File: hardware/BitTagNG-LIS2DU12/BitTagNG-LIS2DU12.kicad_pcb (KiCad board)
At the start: 2 copper layers, 17 x 9 mm, 22 parts, among them J201 CONN_02X04, J301 Conn_01x01, J302 Conn_01x01, J303 Conn_01x01, J304 Conn_01x01, J401 CONN_01X02, Q501 Q_NPN_BEC, U1 at25ex321D-UUN, U3 LIS2DW12TR, U302 stm32l431kc, U501 RV-3028-C7

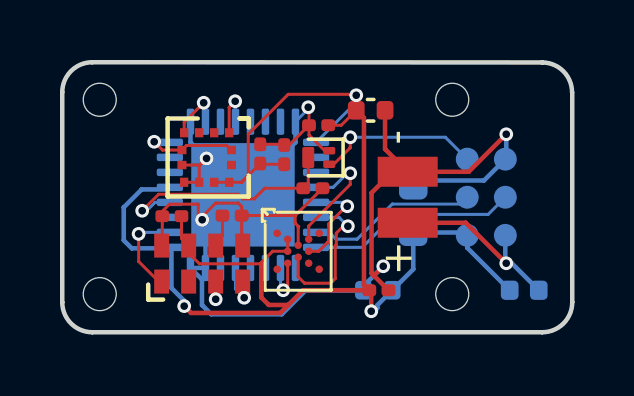
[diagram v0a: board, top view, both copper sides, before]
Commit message: update design
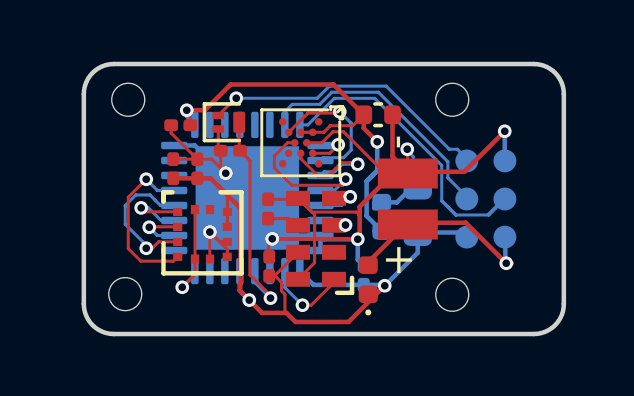
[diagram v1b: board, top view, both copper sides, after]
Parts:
- C4, D401: moved to F.Cu
- C404, C501: moved to B.Cu
- moved C4 5.85 mm to (149.8, 105.7), turned to 0 degrees
- moved D401 5.21 mm to (149.5, 111.2), turned to 90 degrees
- moved C503 4.98 mm to (146.2, 110.7), turned to 90 degrees
- moved U501 3.88 mm to (147.7, 109.8), turned to 180 degrees
- moved U1 3.62 mm to (147.2, 106.6), turned to -90 degrees
- moved C404 3.57 mm to (149.9, 109.1), turned to 90 degrees
- moved Q501 3.22 mm to (144.8, 105.9), turned to 0 degrees
- moved C2 3.04 mm to (143.2, 106.0)
- moved C502 3.02 mm to (144.9, 106.9), turned to 180 degrees
- moved C1 2.94 mm to (143.0, 107.5)
- moved C3 2.94 mm to (143.8, 107.5)
- moved U3 2.56 mm to (144.0, 109.7), turned to 0 degrees
- moved R1 1.22 mm to (146.1, 108.8), turned to 90 degrees
- moved J304 0.95 mm to (141.5, 105.2)
- moved J303 0.85 mm to (141.4, 111.7)
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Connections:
- U3 pad 1: /ACCEL_SCL -> /ACCEL_SCK
- U3 pad 2: unconnected-(U3-CS-Pad2) -> /ACCEL_CS
- U3 pad 3: unconnected-(U3-SDO/SA0-Pad3) -> /ACCEL_MISO
- U3 pad 4: /ACCEL_SDA -> /ACCEL_MOSI
- U302 pad 10: /ACCEL_SDA -> /ACCEL_CS
- U302 pad 11: unconnected-(U302-PA5-Pad11) -> /ACCEL_SCK
- U302 pad 12: /ACCEL_SCL -> /ACCEL_MISO
- U302 pad 13: unconnected-(U302-PA7-Pad13) -> /ACCEL_MOSI
- U302 pad 20: /AT25_nCS -> unconnected-(U302-PA10-Pad20)
- U302 pad 21: /AT25_MISO -> unconnected-(U302-PA11-Pad21)
- U302 pad 22: /AT25_MOSI -> unconnected-(U302-PA12-Pad22)
- U302 pad 25: unconnected-(U302-PA15-Pad25) -> /AT25_nCS
- U302 pad 27: unconnected-(U302-PB4-Pad27) -> /AT25_MISO
- U302 pad 28: unconnected-(U302-PB5-Pad28) -> /AT25_MOSI
- U302 pad 9: GND -> unconnected-(U302-PA3-Pad9)
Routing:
- net VIN: track 48.3 -> 40.2 mm, vias 3 -> 4
- net /ACCEL_MOSI: track 0.00 -> 5.53 mm, vias 0 -> 1
- net /ACCEL_MISO: track 0.00 -> 4.78 mm, vias 0 -> 1
- net SWCLK: track 7.16 -> 11.4 mm
- net RST: track 5.76 -> 9.71 mm
- net SWDIO: track 5.71 -> 8.87 mm
- net /AT25_SCK: track 1.74 -> 4.64 mm
- net /ACCEL_SCK: track 0.00 -> 2.55 mm, vias 0 -> 1
- net /AT25_nCS: track 4.11 -> 1.66 mm
- net /ACCEL_SDA: track 2.22 -> 0.00 mm, vias 1 -> 0
- net /ACCEL_CS: track 0.00 -> 1.99 mm, vias 0 -> 1
- net /ACCEL_SCL: track 1.95 -> 0.00 mm, vias 1 -> 0
- net GND: track 52.9 -> 51.9 mm, vias 5 -> 6
- net /AT25_MISO: track 3.37 -> 4.19 mm
- net VBAT: track 6.95 -> 7.73 mm
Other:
- board size 17 x 9 mm -> 16 x 9 mm
